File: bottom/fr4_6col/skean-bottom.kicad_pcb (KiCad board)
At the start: 2 copper layers, 134.2 x 95.3 mm, 9 parts

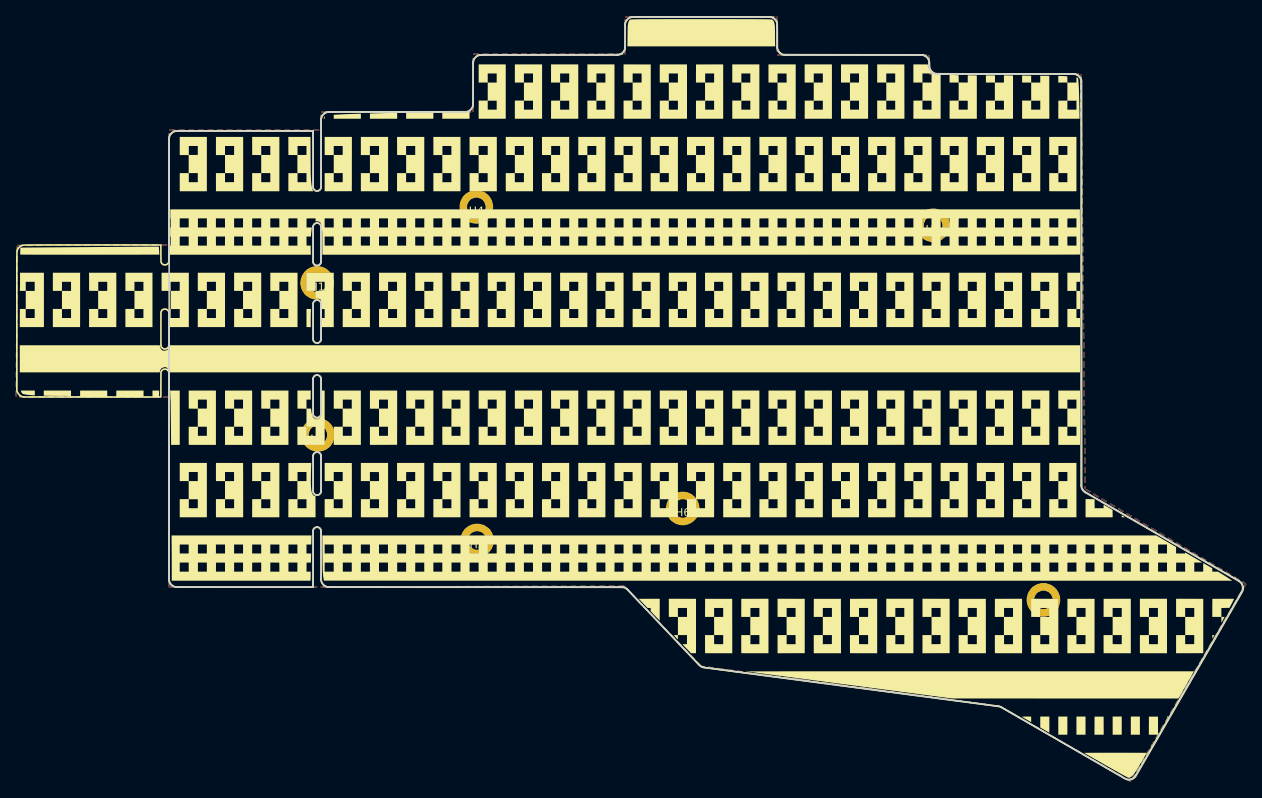
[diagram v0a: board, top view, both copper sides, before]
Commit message: V0.3 case files
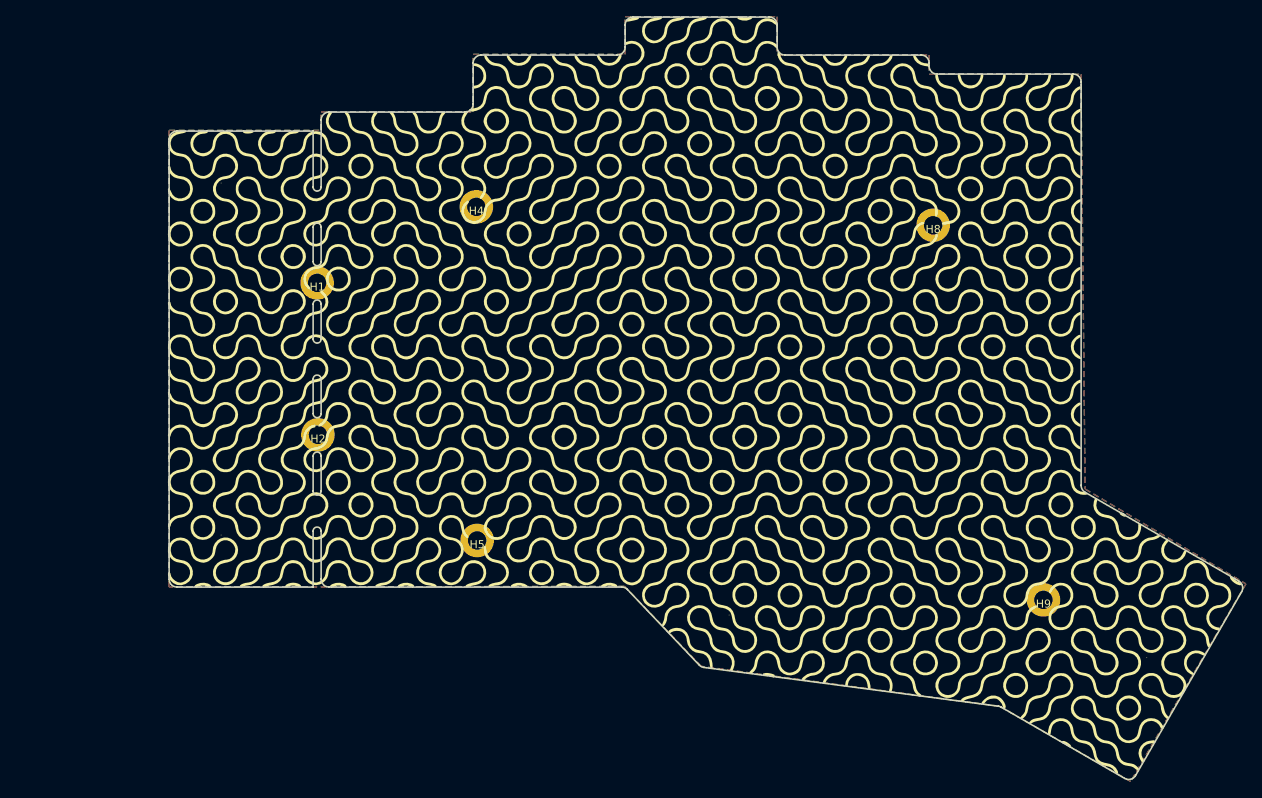
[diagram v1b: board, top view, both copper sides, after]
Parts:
- removed the G*** at (90.8, 62.0) (x2)
- removed H6: MountingHole, kbd:M2_Hole_TH
- added G***: LOGO, Silks:skean_truchet_6col_back, F.Cu at (100.1, 61.6)
- added G***: LOGO, Silks:skean_truchet_6col, F.Cu at (100.1, 61.6)
- added REF**: Bumpon_REV, kbd:Bumpon_REV, F.Cu at (39.7, 35.1)
- added REF**: Bumpon_REV, kbd:Bumpon_REV, F.Cu at (140.7, 28.0)
- added REF**: Bumpon_REV, kbd:Bumpon_REV, F.Cu at (155.4, 94.4)
- added REF**: Bumpon_REV, kbd:Bumpon_REV, F.Cu at (39.7, 79.1)
- added REF**: Bumpon_REV, kbd:Bumpon_REV, F.Cu at (99.7, 20.8)
- added REF**: Bumpon_REV, kbd:Bumpon_REV, F.Cu at (103.2, 89.1)
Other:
- outline, holes or cut-outs redrawn
